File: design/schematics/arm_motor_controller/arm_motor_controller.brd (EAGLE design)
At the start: 97.2 x 54.6 mm, 65 parts, among them Q1 PFET-FQP27P06, Q2 PFET-FQP27P06, Q3 NFET-FQP30N06L, Q4 NFET-FQP30N06L, Q5 PFET-FQP27P06, Q6 PFET-FQP27P06, Q7 NFET-FQP30N06L, Q8 NFET-FQP30N06L

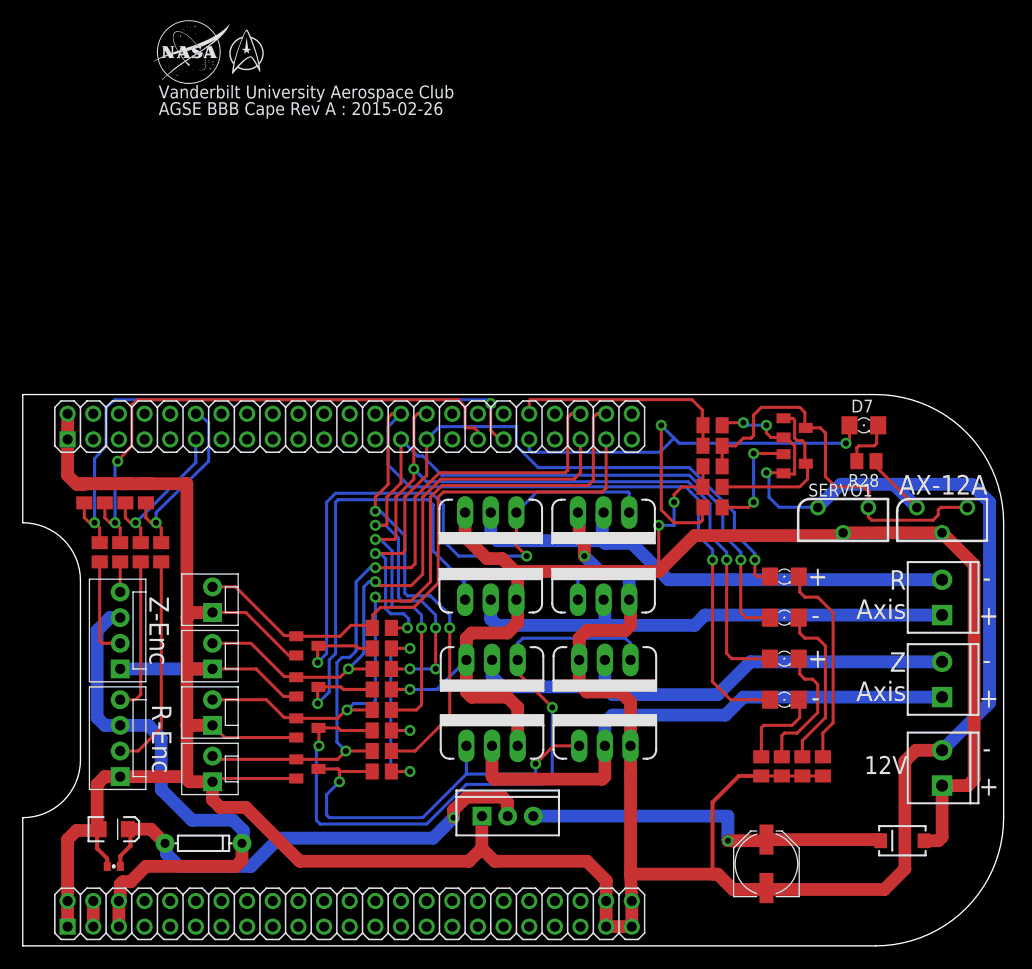
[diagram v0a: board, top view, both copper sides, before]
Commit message: finalizing motor control board.
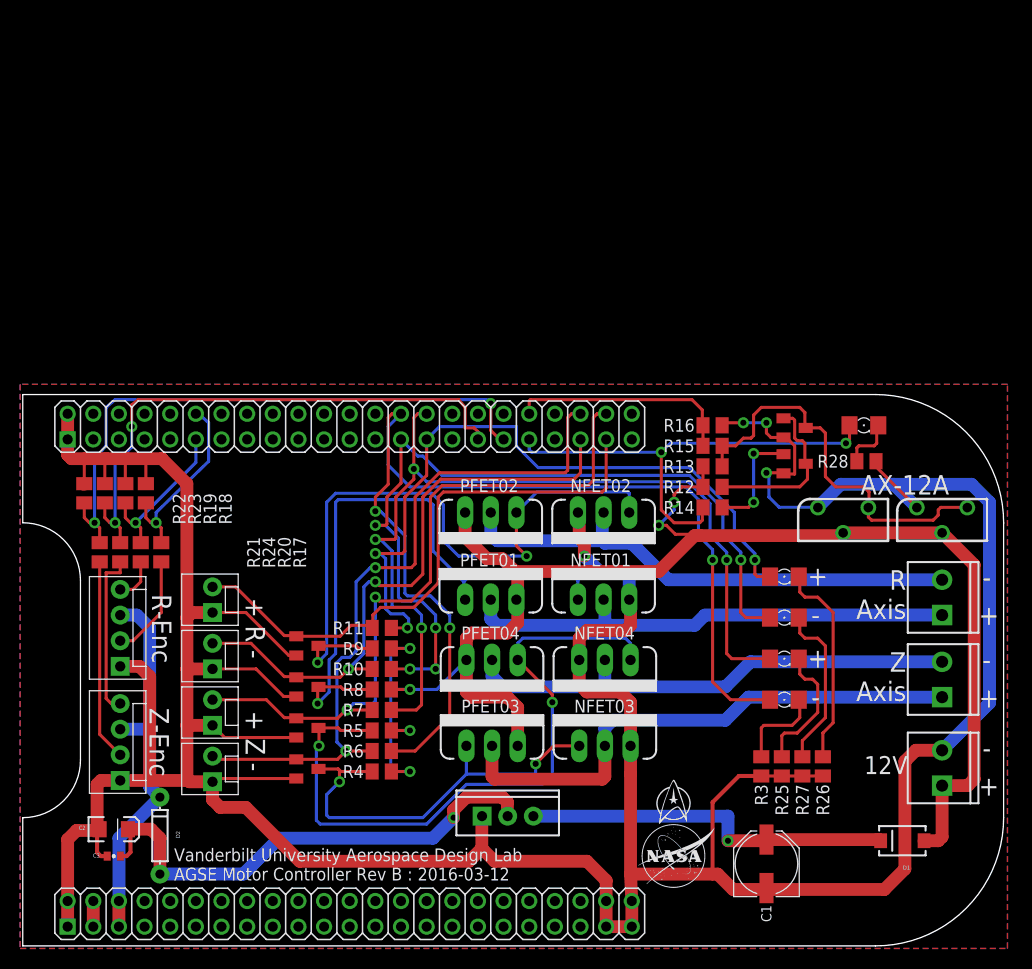
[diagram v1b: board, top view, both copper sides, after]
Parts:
- moved VERTICAL_ENCODER 11.0 mm to (13.7, 16.6)
- moved RADIAL_ENCODER 10.9 mm to (13.7, 27.9)
- moved D2 4.38 mm to (17.7, 11.2), turned to 90 degrees
- moved C3 1.02 mm to (13.1, 9.14)
- renumbered Q1 to PFET01, Q2 to PFET02, Q3 to NFET01, Q4 to NFET02, Q5 to PFET03, Q6 to PFET04, Q7 to NFET03, Q8 to NFET04
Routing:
- net 5V: track 53.8 -> 38.1 mm
- net VERTICAL_ENCODER_B: track 2.99 -> 16.5 mm
- net GND: track 382.3 -> 395.2 mm
- net RADIAL_ENCODER_A: track 21.5 -> 10.2 mm
- net RADIAL_ENCODER_B: track 15.4 -> 4.32 mm
- net VERTICAL_ENCODER_A: track 9.95 -> 20.0 mm
- net BBB_TX: track 51.4 -> 46.5 mm
- net VOUT: track 48.7 -> 50.3 mm
- net 12V: track 163.0 -> 162.1 mm
- net Z-: track 51.0 -> 50.3 mm
- added copper zone on layer 1, net GND
- added copper zone on layer 16, net GND
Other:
- board text added: "+ R -"
- board text added: "+ Z -"
- board text added: "AGSE Motor Controller Rev B : 2016-03-12"
- board text added: "Vanderbilt University Aerospace Design Lab"
- board text removed: "AGSE BBB Cape Rev A : 2015-02-26"
- board text removed: "Vanderbilt University Aerospace Club"

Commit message: finalizing motor controller.
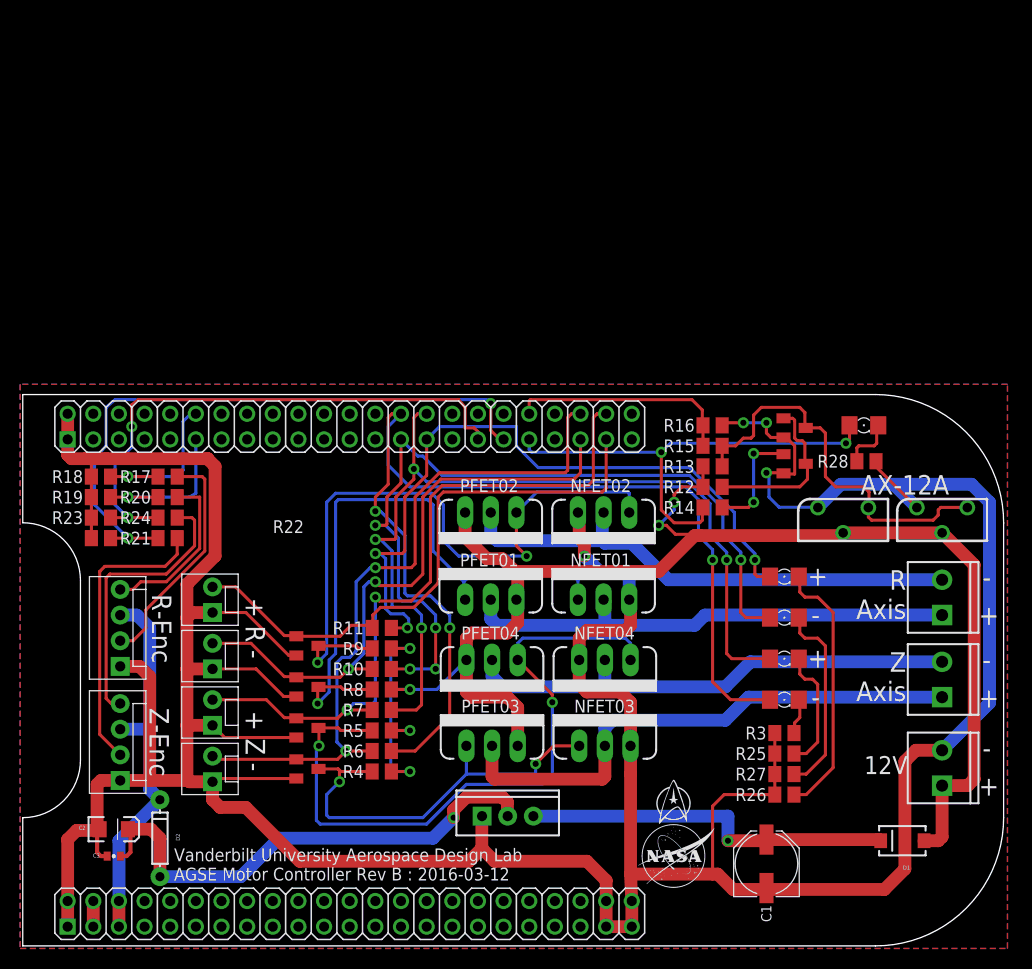
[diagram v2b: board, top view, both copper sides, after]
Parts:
- moved R17 7.52 mm to (18.4, 46.7), turned to 180 degrees
- moved R21 6.87 mm to (18.4, 40.6), turned to 180 degrees
- moved R20 6.08 mm to (18.4, 44.7), turned to 180 degrees
- moved R24 5.82 mm to (18.4, 42.7), turned to 180 degrees
- moved R22 4.74 mm to (11.8, 40.6), turned to 0 degrees
- moved R18 4.74 mm to (11.8, 46.7), turned to 0 degrees
- moved R26 4.72 mm to (79.5, 15.2), turned to 0 degrees
- moved R3 4.02 mm to (79.5, 21.3), turned to 0 degrees
- moved R23 2.44 mm to (11.8, 42.7), turned to 0 degrees
- moved R19 2.44 mm to (11.8, 44.7), turned to 0 degrees
- moved R27 1.93 mm to (79.5, 17.3), turned to 0 degrees
- moved R25 1.30 mm to (79.5, 19.3), turned to 0 degrees
- moved D2 0.25 mm to (17.7, 10.9)
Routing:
- net RADIAL_ENCODER_A: track 10.2 -> 23.1 mm
- net RADIAL_ENCODER_B: track 4.32 -> 16.9 mm
- net VERTICAL_ENCODER_B: track 16.5 -> 28.0 mm
- net VERTICAL_ENCODER_A: track 20.0 -> 29.0 mm
- net N$2: track 20.4 -> 26.1 mm
- net N$5: track 8.91 -> 3.58 mm
- net GND: track 395.2 -> 398.9 mm
- net N$1: track 16.6 -> 19.3 mm
- net BBB_EQEP1A: track 59.7 -> 62.5 mm
- net BBB_EQEP2A: track 18.7 -> 16.8 mm
- net BBB_EQEP2B: track 15.6 -> 16.9 mm
- net N$6: track 13.2 -> 12.3 mm
